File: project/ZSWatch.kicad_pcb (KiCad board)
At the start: 4 copper layers, 41 x 38 mm, 72 parts, among them IC1 APDS-9306-065, IC10 FAN5622SX, IC11 XC9265A331MR-G, IC12 BMP581, IC13 BME688, IC14 LIS2MDLTR, IC15 DRV2603RUNT, IC2 ESDALC6V1W5, IC3 MAX1811ESA+, IC4 DMC2400UV-7, IC5 NCV300LSN36T1G, IC6 AT25SL128A, IC7 XC9265C181MR-G, IC8 BMI270, IC9 NTS0104GU12, M1 NORA-B106, X1 DOCK, X10 M-, X2 BATTERY, X3 GPIO0, X4 GPIO1, X5 GPIO2, X6 GPIO3, X7 GND, X8 GC9A01A_CST816S, X9 M+

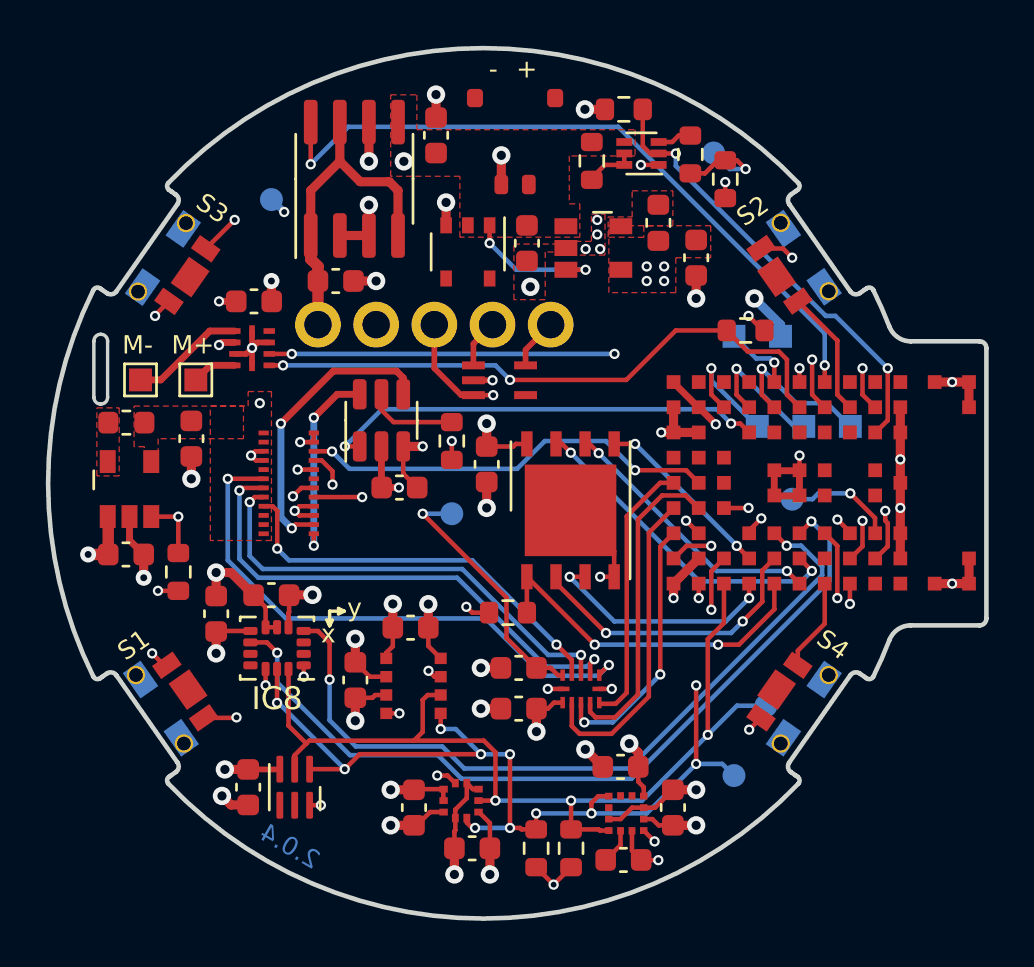
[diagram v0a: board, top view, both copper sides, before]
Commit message: test: fron another repo
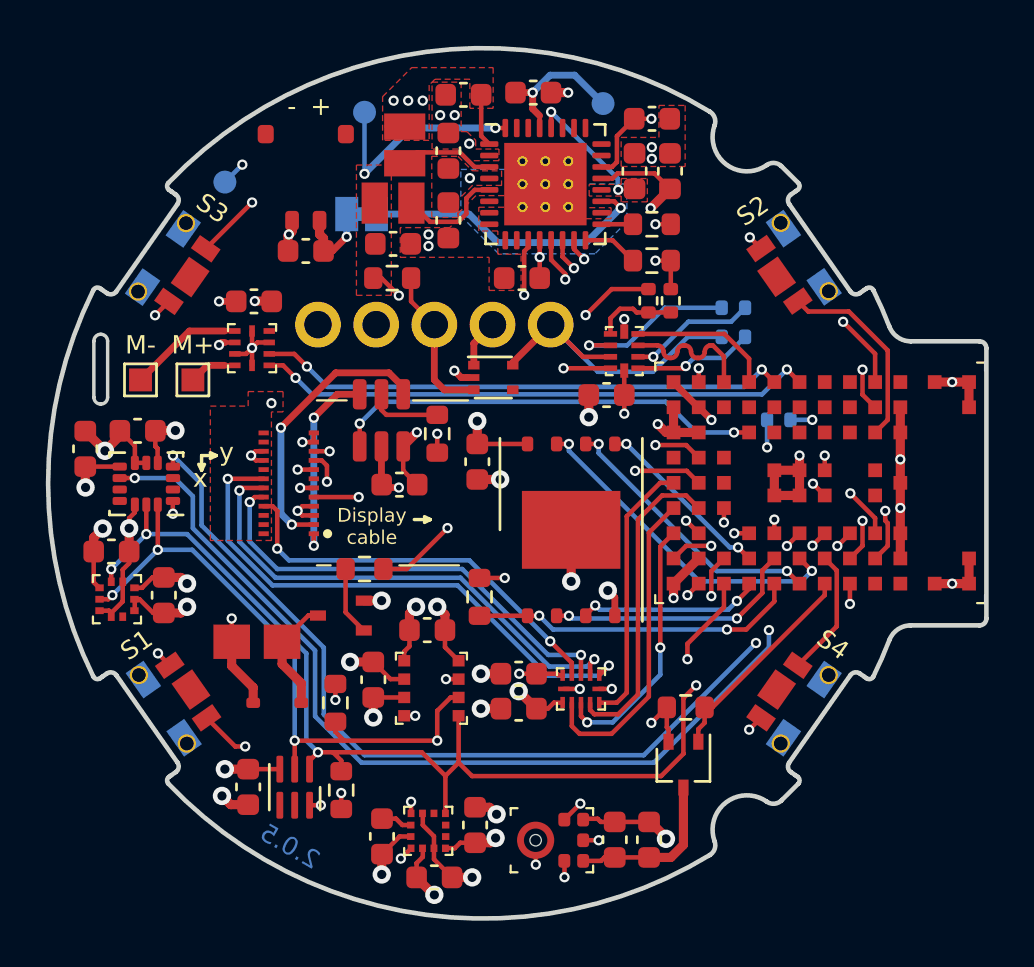
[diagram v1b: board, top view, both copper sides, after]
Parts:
- removed the C11 at (143.8, 115.8)
- removed the C14 at (146.6, 110.8)
- removed the C19 at (156.2, 119.0)
- removed the C21 at (167.6, 126.9)
- removed the IC11 at (143.9, 113.0)
- removed the IC12 at (158.4, 126.6)
- removed IC13: BME688, Package_LGA_Kampi:Bosch_LGA-8_3x3mm_P0.8mm_ClockwisePinNumbering
- removed IC14: LIS2MDLTR, Package_LGA_Kampi:LGA-12_2x2mm_P0.5mm
- removed the IC7 at (164.2, 102.4)
- removed the IC8 at (150.4, 119.9)
- removed the R3 at (169.9, 99.4)
- removed the R5 at (165.5, 96.4)
- removed TP4: 3V3, TestPoint:TestPoint_Pad_D1.0mm
- removed TP5: BAT, TestPoint:TestPoint_Pad_D1.0mm
- removed TP6: 1V8, TestPoint:TestPoint_Pad_D1.0mm
- removed the X2 at (160.8, 97.8)
- removed the X3 at (171.3, 110.2)
- removed the X4 at (173.4, 110.2)
- removed the X5 at (175.4, 110.2)
- removed X6: GPIO3, TestPoint:TestPoint_Pad_1.0x1.0mm
- removed X7: GND, TestPoint:TestPoint_Pad_1.0x1.0mm
- added BZ1: Buzzer, CUI Devices:CMT-322-65-SMT-TR, F.Cu at (149.5, 119.6)
- added C1: 1u, Capacitor_SMD:C_0603_1608Metric, F.Cu at (167.5, 99.1)
- added C10: 1u, Capacitor_SMD:C_0603_1608Metric, F.Cu at (166.7, 96.8)
- added C17: 10u, Capacitor_SMD:C_0603_1608Metric, F.Cu at (159.0, 127.6)
- added C20: 100n, Capacitor_SMD:C_0603_1608Metric, F.Cu at (156.9, 119.1)
- added C23: 1u, Capacitor_SMD:C_0603_1608Metric, F.Cu at (165.1, 128.3)
- added C24: 200p, Capacitor_SMD:C_0603_1608Metric, F.Cu at (166.6, 128.3)
- added C25: 100n, Capacitor_SMD:C_0603_1608Metric, F.Cu at (164.7, 108.9)
- added C5: 10u, Capacitor_SMD:C_0603_1608Metric, F.Cu at (155.4, 102.3)
- added C7: 10u, Capacitor_SMD:C_0603_1608Metric, F.Cu at (158.5, 95.8)
- added C8: 10u, Capacitor_SMD:C_0603_1608Metric, F.Cu at (161.5, 95.7)
- added C9: 10u, Capacitor_SMD:C_0603_1608Metric, F.Cu at (166.0, 99.1)
- added D1: BAS316, Diode_SMD:D_SOD-323, F.Cu at (150.4, 122.3)
- added G***: LOGO, project:QR-Code, B.Cu at (177.0, 112.6)
- added IC1: nPM1300-QEXX, Package_DFN_QFN:QFN-32-1EP_5x5mm_P0.5mm_EP3.6x3.6mm_ThermalVias, F.Cu at (162.1, 99.7)
- added IC10: TS3USB221A, Package_QFN:UQFN-10_1.55x2.05mm_P0.5mm, F.Cu at (165.5, 106.9)
- added IC6: BME688, Package_LGA_Kampi:Bosch_LGA-8_3x3mm_P0.8mm_ClockwisePinNumbering, F.Cu at (157.1, 121.7)
- added J1: ~, Jumper:SolderJumper-2_P1.3mm_Bridged_Pad1.0x1.5mm, B.Cu at (154.1, 101.0)
- added MK1: SPH0645LM4H-B, Knowles:SPH0645LM4H-6_3.5x2.65mm, F.Cu at (162.4, 128.3)
- added Q1: BC817W, Package_TO_SOT_SMD:SOT-323_SC-70, F.Cu at (153.1, 118.5)
- added Q3: DMG1013UW-7, Package_TO_SOT_SMD:SOT-323_SC-70, F.Cu at (168.1, 125.0)
- added R10: 0R, Resistor_SMD:R_0402_1005Metric, F.Cu at (166.6, 104.7)
- added R12: 0R, Resistor_SMD:R_0402_1005Metric, B.Cu at (170.3, 106.3)
- added R13: 0R, Resistor_SMD:R_0402_1005Metric, F.Cu at (167.5, 104.7)
- added R14: 150k, Resistor_SMD:R_0603_1608Metric, F.Cu at (168.2, 122.5)
- added R7: 180R, Resistor_SMD:R_0603_1608Metric, F.Cu at (154.2, 116.5)
- added R8: 100k, Resistor_SMD:R_0603_1608Metric, F.Cu at (155.4, 103.8)
- added X1: BATTERY, Molex:78171-0002, F.Cu at (151.6, 99.4)
- added kibuzzard-656642B5: G***, kibuzzard-656642B5, B.Cu at (152.0, 110.5)
- added kibuzzard-656642E4: G***, kibuzzard-656642E4, B.Cu at (154.7, 110.9)
- added kibuzzard-65664307: G***, kibuzzard-65664307, B.Cu at (157.2, 111.6)
- added kibuzzard-65664337: G***, kibuzzard-65664337, B.Cu at (159.8, 111.6)
- added kibuzzard-65664342: G***, kibuzzard-65664342, B.Cu at (162.3, 111.6)
- C18: value 10u -> 100n
- C2: value 4u7 -> 100n
- C6: value 22u -> 10u
- IC2: renamed from IC1; footprint OptoDevice:Broadcom_DFN-6_2x2mm_P0.65mm -> Broadcom:Broadcom_DFN-6_2x2mm_P0.65mm
- IC3: value MAX1811ESA+ -> BMI270; footprint Package_SO:SOIC-8_3.9x4.9mm_P1.27mm -> Package_LGA:LGA-14_3x2.5mm_P0.5mm_LayoutBorder3x4y
- IC4: value DMC2400UV-7 -> BMP581; footprint Package_TO_SOT_SMD:SOT-563 -> Package_LGA_Kampi:Bosch_LGA-10_2x2mm_P0.5mm_ClockwisePinNumbering
- IC5: value NCV300LSN36T1G -> LIS2MDLTR; footprint Package_SO:TSOP-5_1.65x3.05mm_P0.95mm -> Package_LGA_Kampi:LGA-12_2x2mm_P0.5mm
- IC7: renamed from IC2; footprint Package_SOT_SMD:SOT-325-5 -> Package_TO_SOT_SMD:SOT-665
- IC9: renamed from IC6; value AT25SL128A -> S25FS512SAGNFI010; footprint Package_DFN_QFN:DFN-8-1EP_6x5mm_P1.27mm_EP4x4mm -> Package_SON:WSON-8-1EP_8x6mm_P1.27mm_EP3.4x4.3mm
- L1, L2: value 10u -> 2u2; footprint Inductor_SMD:L_0603_1608Metric -> Inductor_SMD_Kampi:L_0806_2016
- R1: value 1M -> 47k
- R11, R9: value 100k -> 0R; footprint Resistor_SMD:R_0603_1608Metric -> Resistor_SMD:R_0402_1005Metric; moved to B.Cu
- R2: value 1M5 / 0.1% -> 150k
- R3: renamed from R12; value 10k -> 12k
- TP1: value RESET -> 3V3
- TP2: value SCL -> 1V8
- TP3: value SDA -> 3V0
- moved TP2 34.1 mm to (148.1, 99.6), turned to -90 degrees
- moved TP3 31.3 mm to (154.2, 96.5)
- moved IC4 30.0 mm to (143.4, 117.8), turned to 0 degrees
- moved R9 27.0 mm to (172.3, 109.9), turned to 0 degrees
- moved IC5 25.3 mm to (157.0, 127.9)
- moved C15 20.4 mm to (143.1, 115.7), turned to 180 degrees
- moved TP1 19.1 mm to (164.6, 96.1)
- moved L2 17.2 mm to (155.9, 97.9), turned to -90 degrees
- moved IC3 16.1 mm to (144.7, 112.7), turned to 180 degrees
- moved C14 14.3 mm to (145.4, 117.6), turned to 90 degrees
- moved R6 12.1 mm to (152.9, 122.3), turned to 90 degrees
- moved L1 11.6 mm to (155.4, 100.5), turned to 0 degrees
- moved C18 11.4 mm to (154.6, 121.3), turned to 90 degrees
- moved C6 10.9 mm to (157.8, 101.2)
- moved C16 10.6 mm to (154.9, 128.1), turned to -90 degrees
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- renumbered C7 to C11, C1 to C12, C8 to C13, C13 to C14, C17 to C19, C12 to C21, C5 to C22, C9 to C26, C10 to C27, C20 to C28, IC9 to IC11, IC15 to IC12, IC10 to IC8, R6 to R4, R7 to R5, R8 to R6, X1 to X2, X8 to X3, X9 to X4, X10 to X5
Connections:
- C16 pad 1: Net-(IC14-C1) -> Net-(IC5-C1)
- C2 pad 1: VBUS -> +1V8
- C21 pad 2: DISPLAY_3V3 -> /MCU/VDD-Display
- C27 pad 1: DISPLAY_3V3 -> /MCU/VDD-Display
- C28 pad 1: +BATT -> /MCU/VBAT
- C3 pad 1: GND -> /MCU/VBAT
- C3 pad 2: +BATT -> GND
- C4 pad 1: +BATT -> VSYS
- C6 pad 1: +1V8 -> VSYS
- IC11 pad 11: DISPLAY_3V3 -> /MCU/VDD-Display
- IC12 pad 4: unconnected-(IC15-NC-Pad4) -> (no net)
- IC12 pad 7: +BATT -> /MCU/VBAT
- IC2 pad 1: SENSOR_SCL -> /MCU/SENSOR-SCL
- IC2 pad 2: SENSOR_SDA -> /MCU/SENSOR-SDA
- IC3 pad 1: VBUS -> GND
- IC3 pad 2: GND -> unconnected-(IC3-ASDX-Pad2)
- IC3 pad 3: GND -> unconnected-(IC3-ASCX-Pad3)
- IC3 pad 4: VBUS -> /MCU/BMI270-INT1
- IC3 pad 5: +BATT -> +1V8
- IC3 pad 7: VBUS -> GND
- IC3 pad 8: CHG -> +1V8
- IC4 pad 1: GND -> +1V8
- IC4 pad 2: BAT_MON_EN -> /MCU/SENSOR-SCL
- IC4 pad 3: Net-(IC4-D2) -> GND
- IC4 pad 4: +BATT -> /MCU/SENSOR-SDA
- IC4 pad 5: Net-(IC4-D1) -> +1V8
- IC4 pad 6: Net-(IC4-D1) -> +1V8
- IC5 pad 1: Net-(IC5-~{RESET}) -> /MCU/SENSOR-SCL
- IC5 pad 2: +BATT -> unconnected-(IC5-NC-Pad2)
- IC5 pad 3: GND -> +1V8
- IC5 pad 4: (no net) -> /MCU/SENSOR-SDA
- IC5 pad 5: (no net) -> Net-(IC5-C1)
- IC7 pad 1: SWDIO -> D-/SWDIO
- IC7 pad 3: RESETn -> SEL_SWD
- IC7 pad 5: SWDCLK -> D+/SWDCLK
- IC8 pad 3: DISPLAY_3V3 -> /MCU/VDD-Display
- L1 pad 1: Net-(IC7-LX) -> +3V0
- L1 pad 2: +1V8 -> Net-(IC1-SW2)
- L2 pad 1: Net-(IC11-LX) -> +1V8
- L2 pad 2: DISPLAY_3V3 -> Net-(IC1-SW1)
- M1 pad B6: unconnected-(M1B-P0.01/XL2-PadB6) -> BUZZER
- M1 pad B9: unconnected-(M1A-VBUS-PadB9) -> /MCU/VBUS-MCU
- M1 pad C1: SENSOR_SDA -> /MCU/SENSOR-SDA
- M1 pad C8: GPIO0 -> unconnected-(M1B-P0.22-PadC8)
- M1 pad C9: unconnected-(M1A-D+-PadC9) -> MCU_D_P
- M1 pad D3: SENSOR_SCL -> /MCU/SENSOR-SCL
- M1 pad D8: GPIO1 -> unconnected-(M1B-P0.04/AIN0-PadD8)
- M1 pad D9: unconnected-(M1A-D--PadD9) -> MCU_D_N
- M1 pad E3: INT1_LIS -> /MCU/MIC_SEL
- M1 pad E8: GPIO2 -> unconnected-(M1B-P0.05/AIN1-PadE8)
- M1 pad E9: GPIO3 -> DRV_VIB_PWM
- M1 pad F3: INT2_LIS -> /MCU/MIC_DATA
- M1 pad F8: DRV_VIB_EN -> unconnected-(M1C-P1.14-PadF8)
- M1 pad F9: DRV_VIB_PWM -> DRV_VIB_EN
- M1 pad G1: BTN_4 -> /MCU/MIC_EN
- M1 pad G2: unconnected-(M1B-P0.26/AIN5-PadG2) -> BTN_4
- M1 pad G3: BMP581_INT -> /MCU/MIC_BCLK
- M1 pad G4: unconnected-(M1C-P1.04-PadG4) -> /MCU/BMI270-INT2
- M1 pad G5: unconnected-(M1C-P1.08-PadG5) -> /MCU/BMI270-INT1
- M1 pad G8: BTN_3 -> unconnected-(M1C-P1.12-PadG8)
- M1 pad G9: CHG -> unconnected-(M1C-P1.13-PadG9)
- M1 pad H1: LIS2MDL_INT -> /MCU/LIS2MDL_INT
- M1 pad H2: SWDIO -> MCU_SWDIO
- M1 pad H8: BTN_2 -> unconnected-(M1B-P0.30-PadH8)
- M1 pad J2: SWDCLK -> MCU_SWDCLK
- M1 pad J7: BAT_MON_EN -> BTN_2
- M1 pad J8: BAT_MON -> /MCU/PMIC-INT
- M1 pad J9: unconnected-(M1B-P0.31-PadJ9) -> BTN_3
- R1 pad 1: +BATT -> GND
- R1 pad 2: Net-(IC4-D1) -> Net-(IC1-VSET1)
- R11 pad 1: DRV_VIB_EN -> MCU_SWDIO
- R11 pad 2: GND -> D-/SWDIO
- R2 pad 1: Net-(IC4-D2) -> GND
- R2 pad 2: BAT_MON -> Net-(IC1-VSET2)
- R5 pad 1: SENSOR_SCL -> /MCU/SENSOR-SCL
- R6 pad 1: SENSOR_SDA -> /MCU/SENSOR-SDA
- R9 pad 1: DISPLAY_EN -> SEL_SWD
- R9 pad 2: GND -> RESETn
- TP1 pad 1: RESETn -> /MCU/VDD-Display
- TP2 pad 1: SENSOR_SCL -> +1V8
- TP3 pad 1: SENSOR_SDA -> +3V0
- X2 pad 1: SWDCLK -> D+/SWDCLK
- X2 pad 2: SWDIO -> D-/SWDIO
- X2 pad 3: RESETn -> SEL_SWD
- X3 pad 13: DISPLAY_3V3 -> /MCU/VDD-Display
- X3 pad 14: DISPLAY_3V3 -> /MCU/VDD-Display
- X3 pad 17: DISPLAY_3V3 -> /MCU/VDD-Display
- X3 pad 22: unconnected-(X8-NC-Pad22) -> (no net)
- X3 pad 23: DISPLAY_3V3 -> /MCU/VDD-Display
- X3 pad 24: DISPLAY_3V3 -> /MCU/VDD-Display
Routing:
- net /MCU/SENSOR-SCL: track 0.00 -> 82.5 mm, vias 0 -> 6
- net /MCU/SENSOR-SDA: track 0.00 -> 78.4 mm, vias 0 -> 7
- net +3V0: track 0.00 -> 58.8 mm, vias 0 -> 6
- net /MCU/VDD-Display: track 0.00 -> 51.9 mm, vias 0 -> 4
- net SENSOR_SCL: track 48.7 -> 0.00 mm, vias 12 -> 0
- net /MCU/BMI270-INT2: track 0.00 -> 47.9 mm, vias 0 -> 3
- net /MCU/BMI270-INT1: track 0.00 -> 47.1 mm, vias 0 -> 3
- net SENSOR_SDA: track 42.4 -> 0.00 mm, vias 3 -> 0
- net INT2_LIS: track 35.7 -> 0.00 mm, vias 2 -> 0
- net INT1_LIS: track 33.3 -> 0.00 mm, vias 2 -> 0
- net +BATT: track 32.6 -> 0.00 mm, vias 4 -> 0
- net CHG: track 30.8 -> 0.00 mm, vias 2 -> 0
- net SEL_SWD: track 0.00 -> 26.8 mm, vias 0 -> 2
- net SWDIO: track 26.1 -> 0.00 mm, vias 1 -> 0
- net /MCU/LIS2MDL_INT: track 0.00 -> 25.7 mm, vias 0 -> 2
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- added copper zone on F.Cu, net +3V0
- added copper zone on F.Cu, net /MCU/VDD-Display
- added copper zone on B.Cu, net VSYS
- added copper zone on F.Cu, net VSYS
- removed copper zone on F.Cu, net +BATT
- removed copper zone on F.Cu, net DISPLAY_3V3
- removed copper zone on F.Cu, net Net-(IC11-LX)
- removed copper zone on F.Cu, net Net-(IC7-LX)
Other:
- outline, holes or cut-outs redrawn
- board text added: "Dielektrikum"
- board text added: "Display cable"
- board text added: "Inner1"
- board text added: "Inner2"
- board text removed: "5V"
- board text removed: "Dielektrikum 1"
- board text removed: "Dielektrikum 2"
- board text removed: "Dielektrikum 3"
- board text removed: "GND"
- board text removed: "Layer2"
- board text removed: "Layer3"
- board text removed: "Reset"
- board text removed: "SWDCLK"
- board text removed: "SWDIO"
